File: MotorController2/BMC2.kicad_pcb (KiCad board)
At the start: 2 copper layers, 178.2 x 57.8 mm, 130 parts, among them P1 Sensor, P10 GND, P11 I2C, P12 CAN, P2 CAN, P3 DATA, P4 USB_OTG, P5 PhaseA, P6 PhaseB, P7 PhaseC, P8 CONN_02X05, P9 VSUPPLY, Q1 BSC016N06NS, Q2 BSC016N06NS, Q3 BSC016N06NS, Q4 BSC016N06NS, Q5 BSC016N06NS, Q6 BSC016N06NS, SW1 RESET, SW2 CAL, U1 TJA1042T/3, U2 STM32F205RBTx, U3 DRV8305, U4 IFX91041EJV50, U5 TC2117-3.3V, X1 8MHz

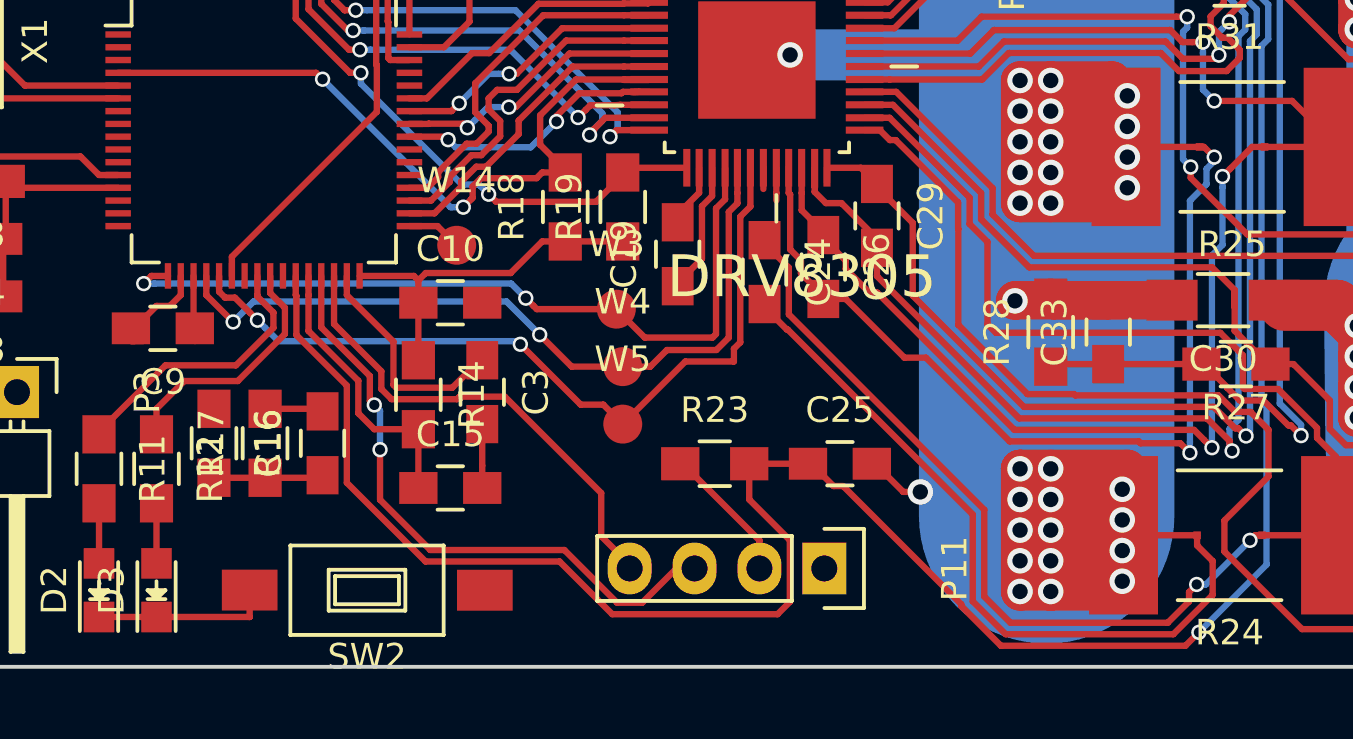
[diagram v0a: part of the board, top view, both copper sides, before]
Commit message: More tweaks
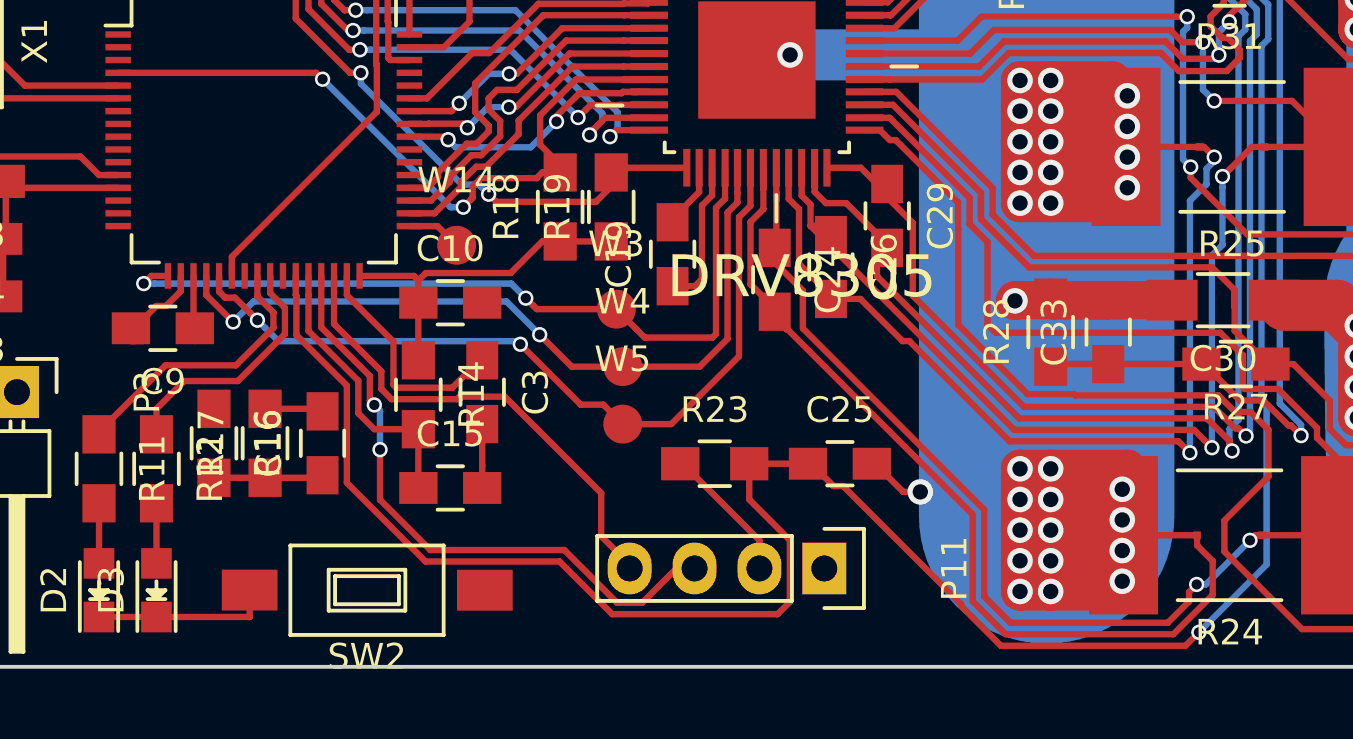
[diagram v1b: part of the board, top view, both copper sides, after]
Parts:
- moved C24 0.50 mm to (186.2, 95.6)
- moved R19 0.45 mm to (179.8, 92.8)
- moved C29 0.40 mm to (190.6, 93.1)
- moved C26 0.30 mm to (188.4, 95.1)
- moved C19 0.20 mm to (182.2, 94.6)
- moved R18 0.20 mm to (177.8, 92.8)
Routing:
- net Net-(C24-Pad2): track 29.0 -> 35.2 mm
- net Net-(C24-Pad1): track 31.7 -> 33.4 mm
- net Net-(C26-Pad1): track 34.8 -> 35.6 mm
- net Net-(C26-Pad2): track 35.8 -> 35.1 mm
- net Net-(C19-Pad1): track 5.19 -> 5.79 mm
